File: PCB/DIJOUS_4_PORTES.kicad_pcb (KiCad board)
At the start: 2 copper layers, 91.2 x 101.1 mm, 66 parts, among them J1 PowerIN, J10 DOOR_LCK, J12 WIN_SW, J14 FINAL_CARRERA_UP, J15 FINAL_CARRERA_DOWN, J2 OUT_WIN, J3 ICSP, J4 CAN, J5 OUT_DOOR, J6 USART, J8 RFID_COAX, SW1 DOOR_LCK, SW3 WIN_SW, U1 LT1528CT-PBF, U2 PIC32MK0256MCJ048-I/Y8X, U3 TCAN334D, U4 MAX22201ATC+, U5 MAX22201ATC+, Y1 ASZKDV-32.768KHZ-L-T3, Y2 ECS-3225SMV-080-GP-TR

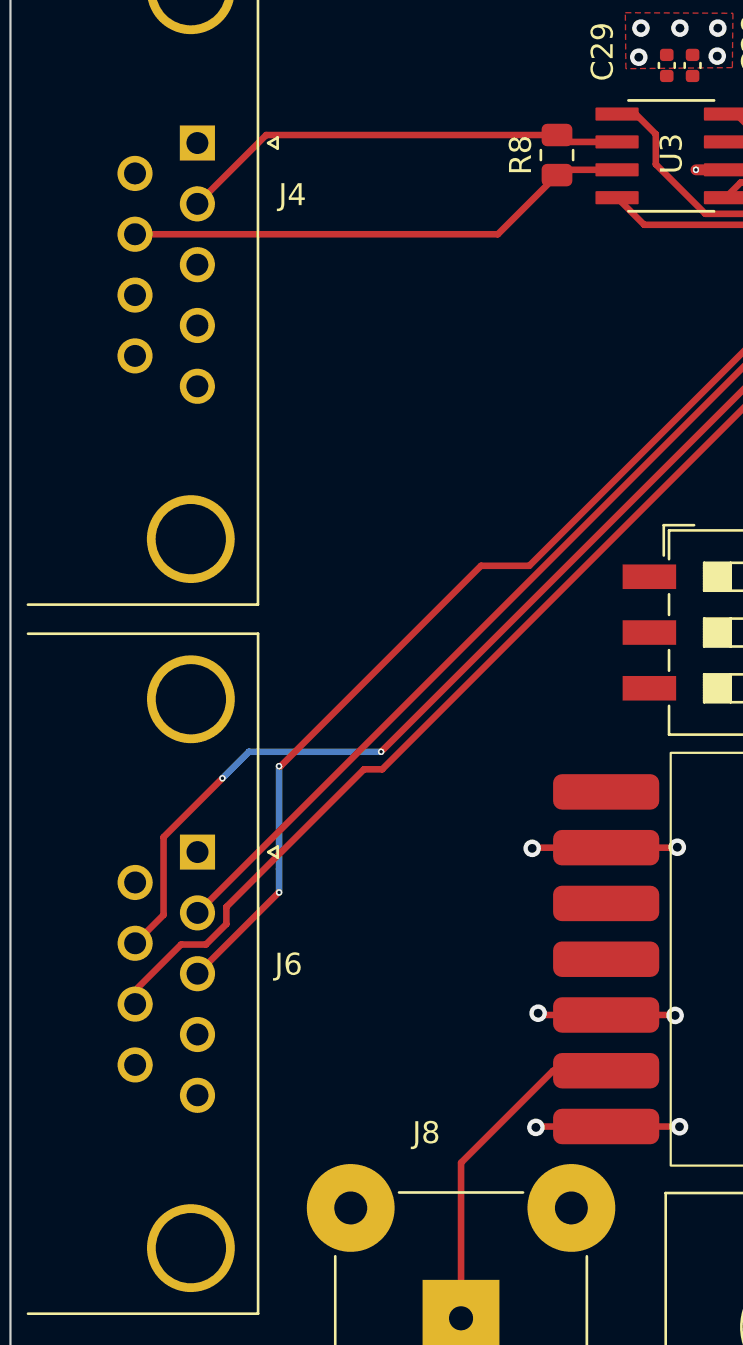
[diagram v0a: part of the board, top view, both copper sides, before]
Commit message: parell diferencial
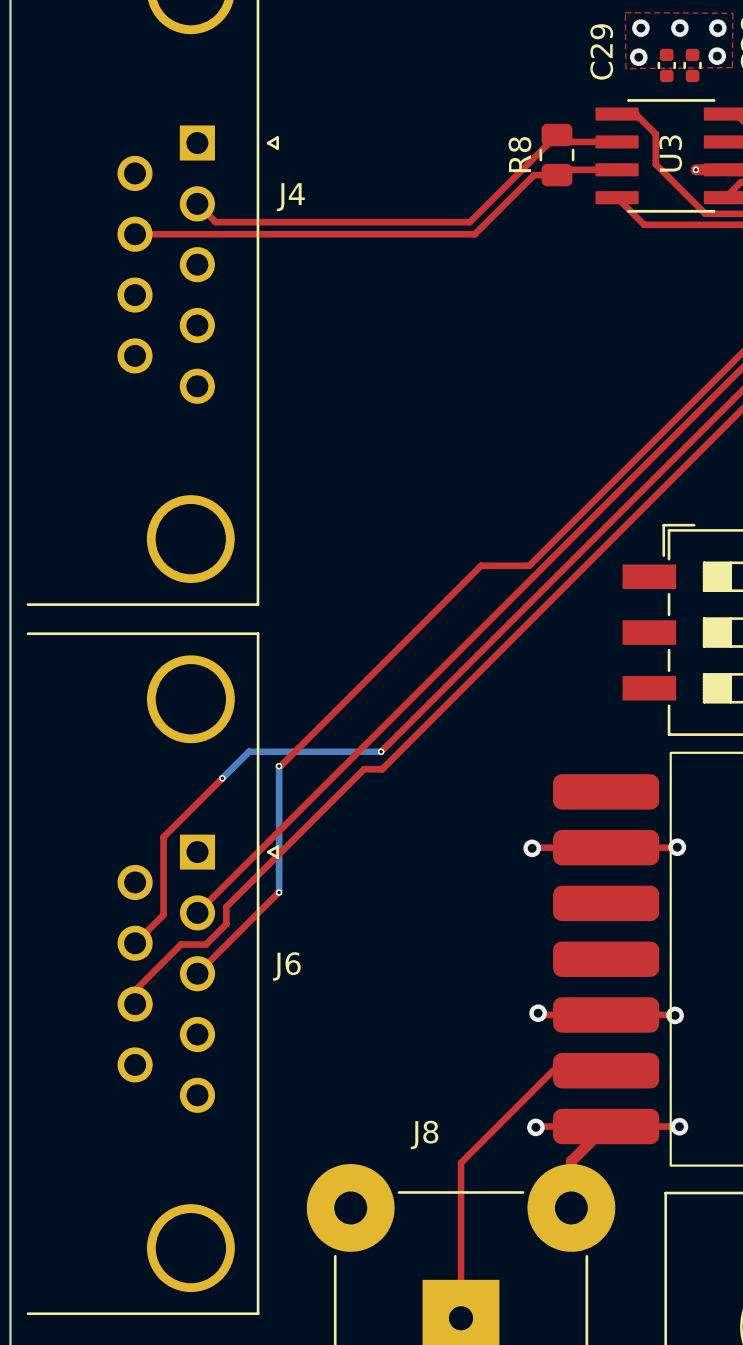
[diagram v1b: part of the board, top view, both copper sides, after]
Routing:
- net GND: track 42.6 -> 46.9 mm
- net CAN_N: track 20.5 -> 21.2 mm
